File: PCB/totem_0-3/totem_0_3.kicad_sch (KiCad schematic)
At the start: 88 parts, among them J1 MJ-4PP-9, J2 MJ-4PP-9, U1 xiao-ble, U2 xiao-ble

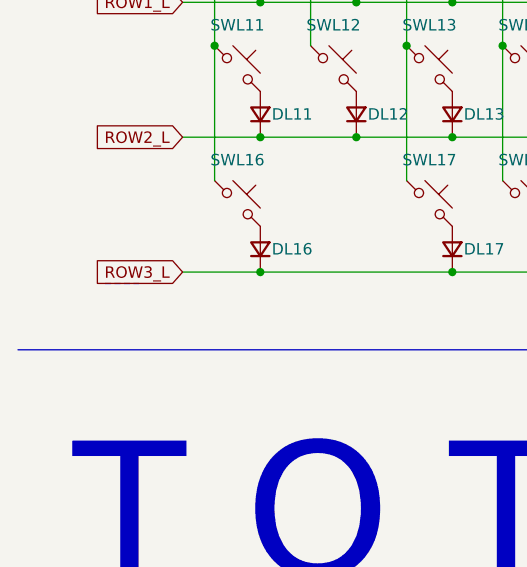
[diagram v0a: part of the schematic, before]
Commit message: production totem 0-4
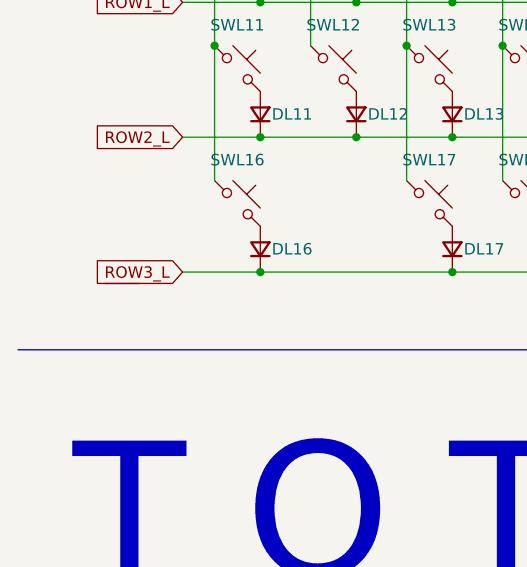
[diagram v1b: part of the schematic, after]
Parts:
- U1, U2: footprint TOTEMlib:XIAO-ble-plus -> TOTEMlib:xiao-ble-smd-cutout

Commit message: intial xiao plus
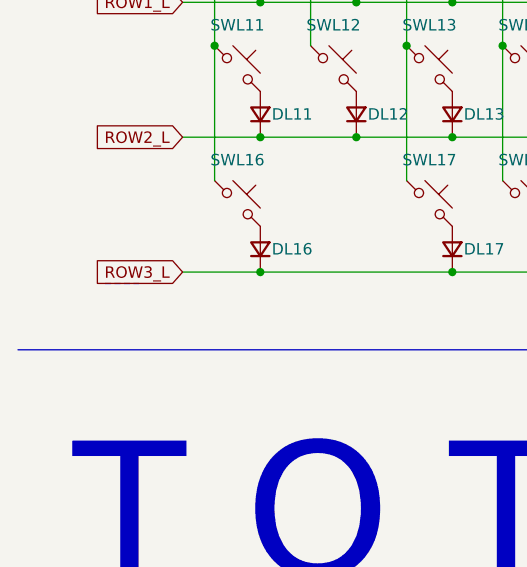
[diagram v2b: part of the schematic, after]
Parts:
- U1, U2: footprint TOTEMlib:xiao-ble-smd-cutout -> TOTEMlib:XIAO-ble-plus
